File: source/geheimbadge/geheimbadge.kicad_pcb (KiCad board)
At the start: 2 copper layers, 75.9 x 74.5 mm, 77 parts, among them J1 SAOv2

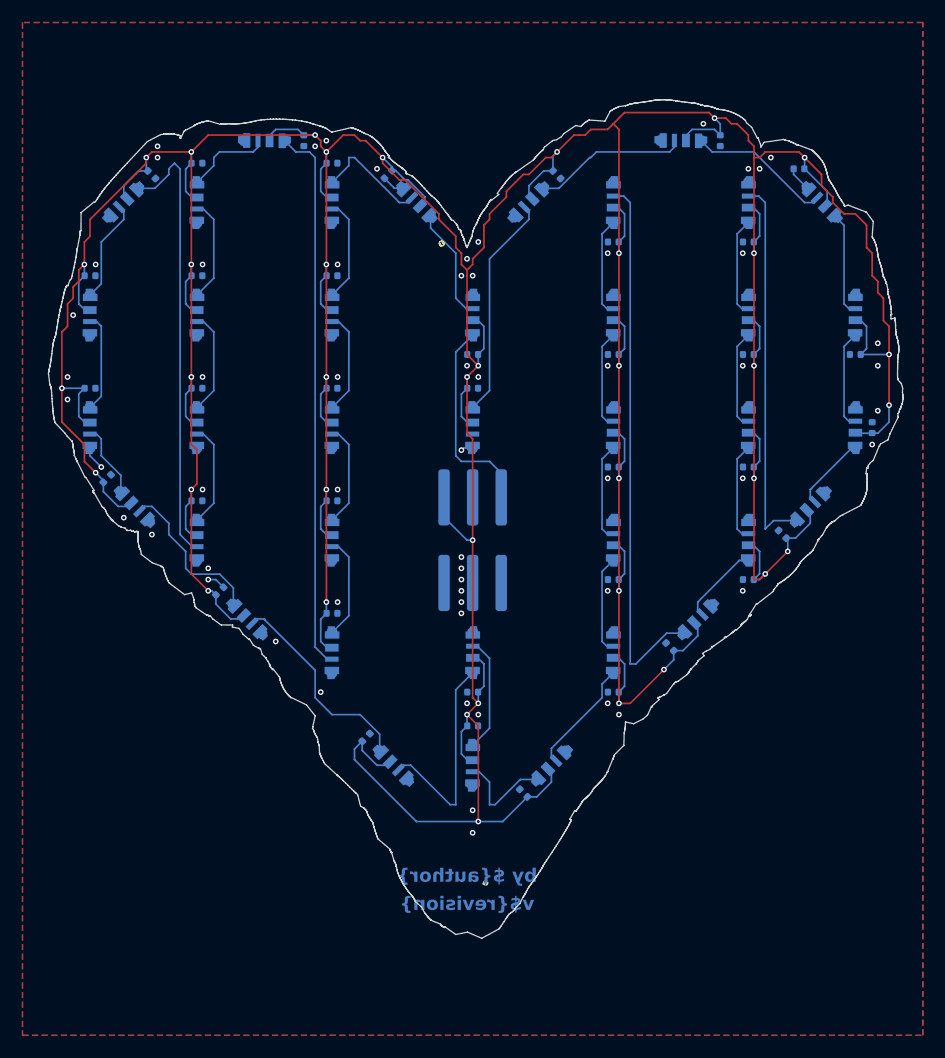
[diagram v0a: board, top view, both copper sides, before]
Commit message: flipped board
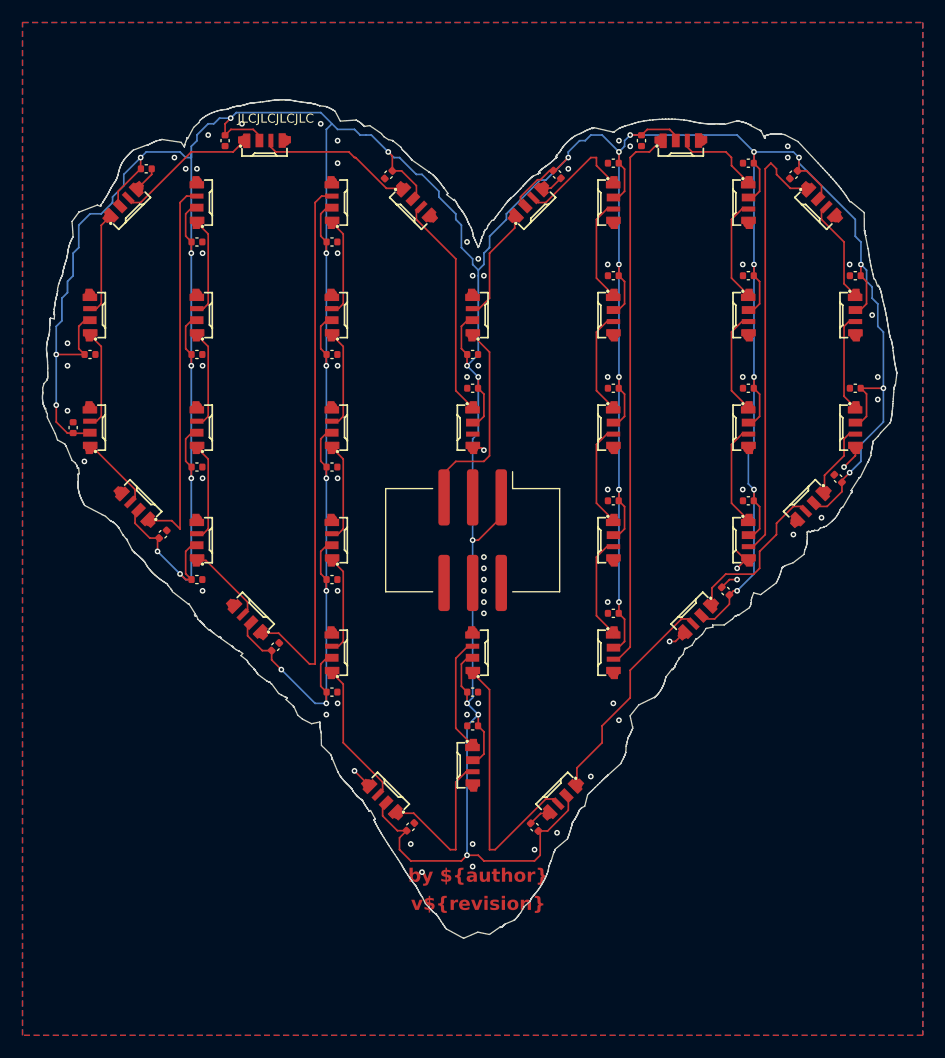
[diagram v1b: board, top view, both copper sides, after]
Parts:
- C1, C10, C11, C12, C13, C14, C15, C16, C17, C18, C19, C2, C20, C21, C22, C23, C24, C25, C26, C27, C28, C29, C3, C30, C31, C32, C33, C34, C35, C36, C37, C38, C4, C5, C6, C7, C8, C9, D1, D10, D11, D12, D13, D14, D15, D16, D17, D18, D19, D2, D20, D21, D22, D23, D24, D25, D26, D27, D28, D29, D3, D30, D31, D32, D33, D34, D35, D36, D37, D38, D4, D5, D6, D7, D8, D9, J1: moved to F.Cu
- moved C33 71.0 mm to (64.5, 116.0)
- moved C14 68.0 mm to (134.0, 102.5), turned to 180 degrees
- moved C15 68.0 mm to (134.0, 112.5), turned to 180 degrees
- moved C34 68.0 mm to (66.0, 109.5), turned to 0 degrees
- moved D14 68.0 mm to (134.0, 106.0)
- moved D15 68.0 mm to (134.0, 116.0)
- moved D33 68.0 mm to (66.0, 116.0)
- moved D34 68.0 mm to (66.0, 106.0)
- moved C16 64.9 mm to (132.5, 120.5), turned to 135 degrees
- moved D13 62.0 mm to (131.0, 96.0), turned to -45 degrees
- moved D35 62.0 mm to (69.0, 96.0), turned to 45 degrees
- moved D16 60.0 mm to (130.0, 123.0), turned to -135 degrees
- moved D32 60.0 mm to (70.0, 123.0), turned to 135 degrees
- moved C35 58.0 mm to (71.0, 93.0), turned to 0 degrees
- moved C13 57.1 mm to (128.5, 93.5), turned to -135 degrees
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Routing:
- net GND: track 9.00 -> 16.9 mm, vias 58 -> 69
- net /pixel19/D_{out}: track 9.04 -> 14.5 mm
- net /pixel17/D_{out}: track 19.0 -> 24.5 mm
- net /pixel20/D_{out}: track 10.2 -> 12.8 mm
- net VCC: track 586.0 -> 587.4 mm
- net /pixel16/D_{out}: track 18.7 -> 19.8 mm
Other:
- outline, holes or cut-outs redrawn

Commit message: finalized controller design
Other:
- board text added: "0, 3"
- board text added: "10"
- board text added: "11, 16"
- board text added: "12"
- board text added: "13"
- board text added: "14, 15"
- board text added: "17"
- board text added: "20"
- board text added: "22"
- board text added: "23"
- board text added: "24"
- board text added: "25"
- board text added: "26, 27"
- board text added: "28"
- board text added: "29"
- board text added: "30, 35"
- board text added: "32, 31"
- board text added: "33"
- board text added: "34"
- board text added: "4"
- board text added: "5"
- board text added: "6, 18"
- board text added: "7, 8"
- board text added: "9"
- board text removed: "10, 15"
- board text removed: "11, 12, 13"
- board text removed: "14"
- board text removed: "16"
- board text removed: "17, 4"
- board text removed: "18, 31"
- board text removed: "19"
- board text removed: "20, 25"
- board text removed: "22, 23, 24"
- board text removed: "26, 30"
- board text removed: "27, 28, 29"
- board text removed: "3"
- board text removed: "32, 36"
- board text removed: "33, 34, 35"
- board text removed: "37"
- board text removed: "38"
- board text removed: "5, 9"
- board text removed: "6, 7, 8"

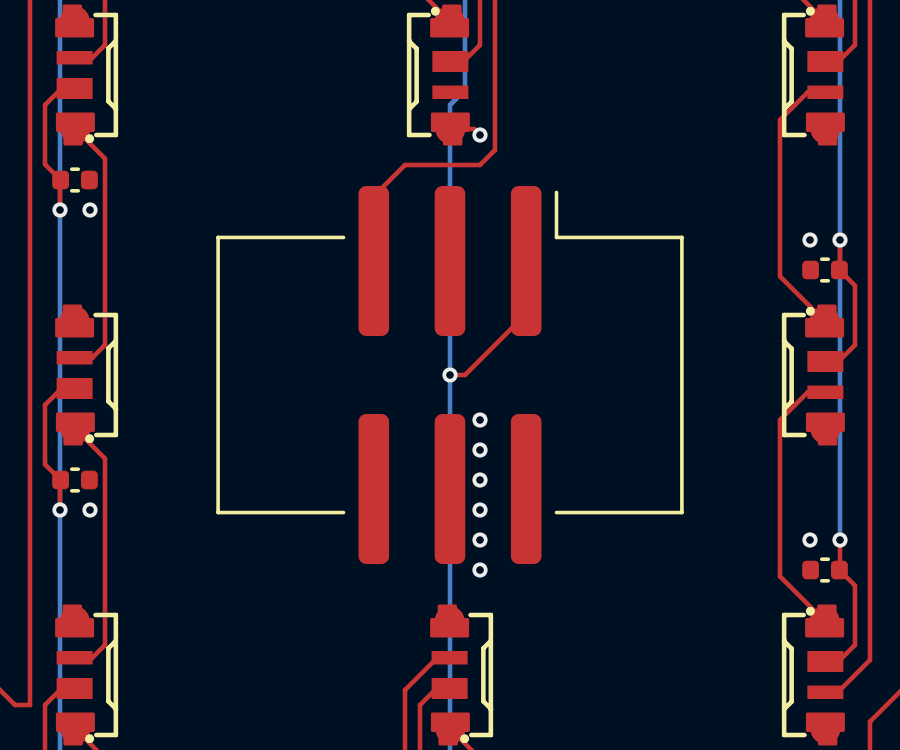
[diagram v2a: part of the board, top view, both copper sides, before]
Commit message: finalized all designs
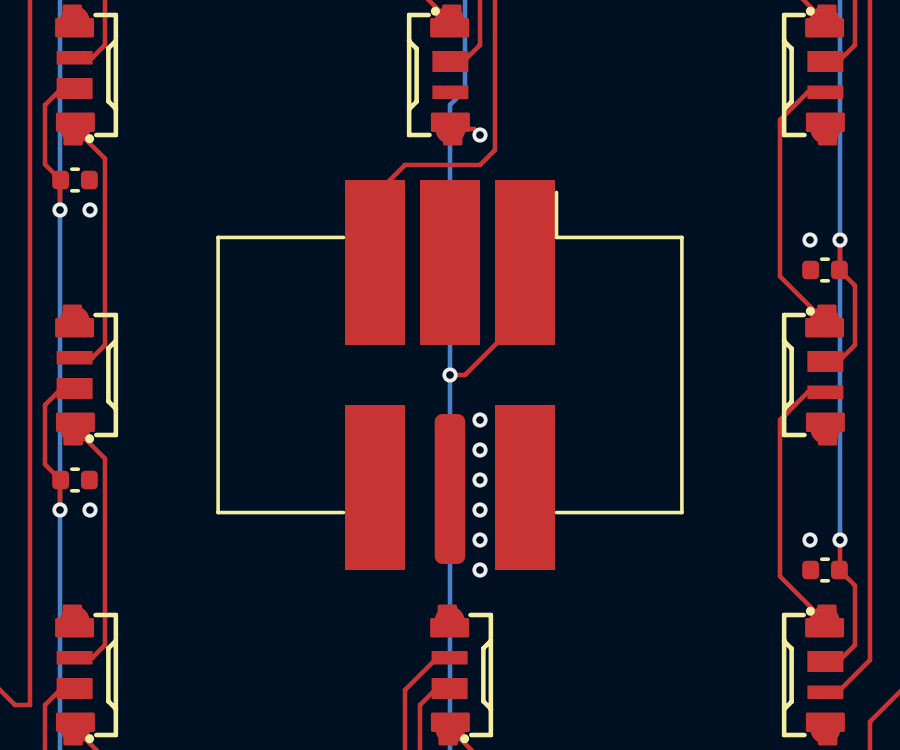
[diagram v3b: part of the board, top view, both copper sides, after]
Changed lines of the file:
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@@
 	(property "company" "Geheimorganisation")
 	(property "pid" "tba")
-	(property "revision" "0.1.1")
+	(property "revision" "1.0.0")
 	(property "title" "Geheimbadge")
 	(net 0 "")
@@
 		)
 	)
+	(gr_rect
+		(start 101.5 119.5)
+		(end 103.5 125)
+		(stroke
+			(width 0)
+			(type solid)
+		)
+		(fill solid)
+		(layer "F.Cu")
+		(net 1)
+	)
+	(gr_rect
+		(start 96.5 127)
+		(end 98.5 132.5)
+		(stroke
+			(width 0)
+			(type solid)
+		)
+		(fill solid)
+		(layer "F.Cu")
+		(net 6)
+	)
+	(gr_rect
+		(start 99 119.5)
+		(end 101 125)
+		(stroke
+			(width 0)
+			(type solid)
+		)
+		(fill solid)
+		(layer "F.Cu")
+		(net 3)
+	)
+	(gr_rect
+		(start 96.5 119.5)
+		(end 98.5 125)
+		(stroke
+			(width 0)
+			(type solid)
+		)
+		(fill solid)
+		(layer "F.Cu")
+		(net 4)
+	)
+	(gr_rect
+		(start 101.5 127)
+		(end 103.5 132.5)
+		(stroke
+			(width 0)
+			(type solid)
+		)
+		(fill solid)
+		(layer "F.Cu")
+		(net 2)
+	)
 	(gr_poly
